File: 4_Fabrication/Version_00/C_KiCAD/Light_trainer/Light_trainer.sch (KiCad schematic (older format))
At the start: 25 parts, among them SW1 SW_Push, SW2 SW_Push, SW3 SW_Push, SW4 SW_Push, U1 LTC3525-5, U2 ESP32-DevKitC-32D

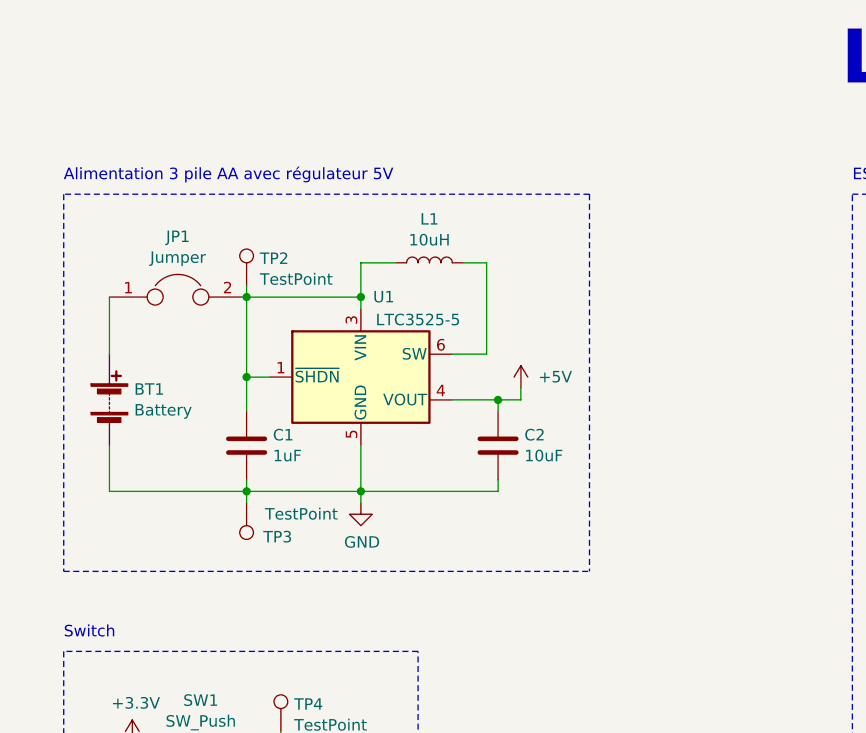
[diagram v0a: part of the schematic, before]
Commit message: placement + routage
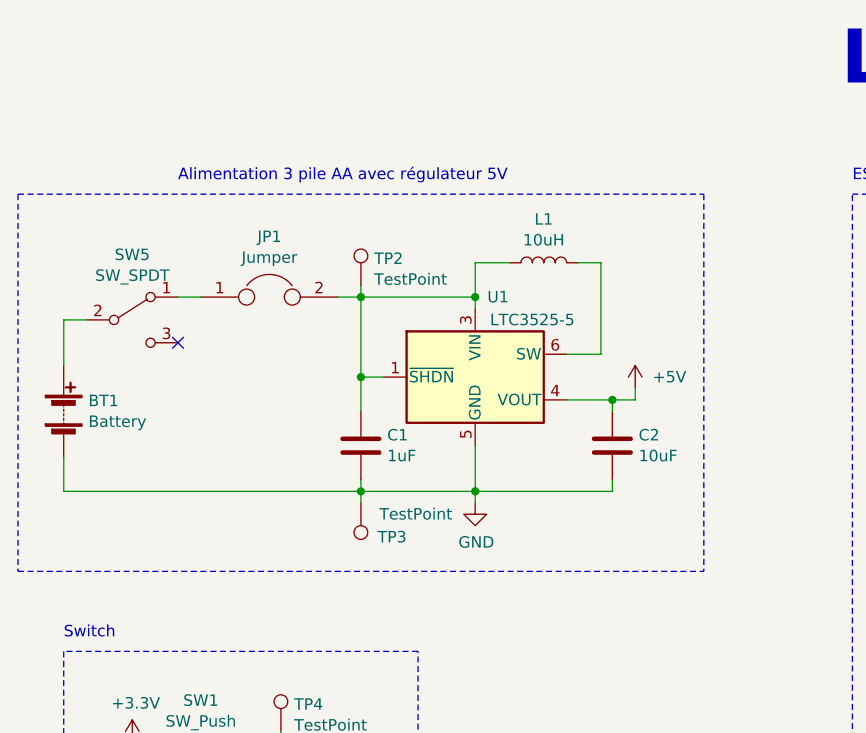
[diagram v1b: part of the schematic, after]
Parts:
- added SW5: SW_SPDT, Work_Forestier:C&K-1101M2S5CQE2, symbol Switch:SW_SPDT
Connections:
- net at BT1.1 (+): now also SW5.2 (B); no longer JP1.1
- new net: JP1.1, SW5.1 (A)
- no-connect marks 31 -> 32
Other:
- moved on the sheet: BT1, C1, C2, JP1, L1, TP2, TP3, U1
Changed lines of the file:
@@
 L Device:Battery BT1
 U 1 1 613C716D
-P 1200 2400
-F 0 "BT1" H 1308 2446 50  0000 L CNN
-F 1 "Battery" H 1308 2355 50  0000 L CNN
-F 2 "Work_Forestier:BatteryHolder_Keystone_2464_3xAA" V 1200 2460 50  0001 C CNN
-F 3 "~" V 1200 2460 50  0001 C CNN
-	1    1200 2400
+P 1000 2450
+F 0 "BT1" H 1108 2496 50  0000 L CNN
+F 1 "Battery" H 1108 2405 50  0000 L CNN
+F 2 "Work_Forestier:BatteryHolder_Keystone_2464_3xAA" V 1000 2510 50  0001 C CNN
+F 3 "~" V 1000 2510 50  0001 C CNN
+	1    1000 2450
 	1    0    0    -1
 $EndComp
@@
 L Regulator_Switching:LTC3525-5 U1
 U 1 1 613E4BD4
-P 2300 2300
-F 0 "U1" H 2400 2650 50  0000 C CNN
-F 1 "LTC3525-5" H 2550 2550 50  0000 C CNN
-F 2 "Package_TO_SOT_SMD:SOT-363_SC-70-6" H 2350 2050 50  0001 L CNN
-F 3 "https://www.analog.com/media/en/technical-documentation/data-sheets/3525fc.pdf" H 2300 2300 50  0001 C CNN
-	1    2300 2300
-	1    0    0    -1
-$EndComp
-Wire Wire Line
-	1800 2300 1900 2300
+P 2800 2300
+F 0 "U1" H 2900 2650 50  0000 C CNN
+F 1 "LTC3525-5" H 3050 2550 50  0000 C CNN
+F 2 "Package_TO_SOT_SMD:SOT-363_SC-70-6" H 2850 2050 50  0001 L CNN
+F 3 "https://www.analog.com/media/en/technical-documentation/data-sheets/3525fc.pdf" H 2800 2300 50  0001 C CNN
+	1    2800 2300
+	1    0    0    -1
+$EndComp
+Wire Wire Line
+	2300 2300 2400 2300
 $Comp
 L Device:L L1
 U 1 1 613E7FA8
-P 2600 1800
-F 0 "L1" V 2790 1800 50  0000 C CNN
-F 1 "10uH" V 2699 1800 50  0000 C CNN
-F 2 "Inductor_SMD:L_1210_3225Metric" H 2600 1800 50  0001 C CNN
-F 3 "~" H 2600 1800 50  0001 C CNN
-	1    2600 1800
+P 3100 1800
+F 0 "L1" V 3290 1800 50  0000 C CNN
+F 1 "10uH" V 3199 1800 50  0000 C CNN
+F 2 "Inductor_SMD:L_1210_3225Metric" H 3100 1800 50  0001 C CNN
+F 3 "~" H 3100 1800 50  0001 C CNN
+	1    3100 1800
 	0    -1   -1   0
 $EndComp
 Wire Wire Line
-	2850 1800 2850 2200
-Wire Wire Line
-	2850 2200 2700 2200
+	3350 1800 3350 2200
+Wire Wire Line
+	3350 2200 3200 2200
 $Comp
 L Device:C C2
 U 1 1 613EB1F1
-P 2900 2600
-F 0 "C2" H 3015 2646 50  0000 L CNN
-F 1 "10uF" H 3015 2555 50  0000 L CNN
-F 2 "Capacitor_SMD:C_0805_2012Metric" H 2938 2450 50  0001 C CNN
-F 3 "~" H 2900 2600 50  0001 C CNN
-	1    2900 2600
-	1    0    0    -1
-$EndComp
-Wire Wire Line
-	2900 2400 2900 2450
-Wire Wire Line
-	2700 2400 2900 2400
-Wire Wire Line
-	2900 2400 3000 2400
-Connection ~ 2900 2400
-Wire Wire Line
-	2300 2600 2300 2800
-Wire Wire Line
-	2300 2800 2900 2800
-Wire Wire Line
-	2900 2800 2900 2750
+P 3400 2600
+F 0 "C2" H 3515 2646 50  0000 L CNN
+F 1 "10uF" H 3515 2555 50  0000 L CNN
+F 2 "Capacitor_SMD:C_0805_2012Metric" H 3438 2450 50  0001 C CNN
+F 3 "~" H 3400 2600 50  0001 C CNN
+	1    3400 2600
+	1    0    0    -1
+$EndComp
+Wire Wire Line
+	3400 2400 3400 2450
+Wire Wire Line
+	3200 2400 3400 2400
+Wire Wire Line
+	3400 2400 3500 2400
+Connection ~ 3400 2400
+Wire Wire Line
+	2800 2600 2800 2800
+Wire Wire Line
+	2800 2800 3400 2800
+Wire Wire Line
+	3400 2800 3400 2750
 $Comp
 L Device:C C1
 U 1 1 613F1363
-P 1800 2600
-F 0 "C1" H 1915 2646 50  0000 L CNN
-F 1 "1uF" H 1915 2555 50  0000 L CNN
-F 2 "Capacitor_SMD:C_0805_2012Metric" H 1838 2450 50  0001 C CNN
-F 3 "~" H 1800 2600 50  0001 C CNN
-	1    1800 2600
-	1    0    0    -1
-$EndComp
-Wire Wire Line
-	2300 2800 1800 2800
-Wire Wire Line
-	1800 2800 1800 2750
-Connection ~ 2300 2800
-Wire Wire Line
-	1800 2450 1800 2300
-Wire Wire Line
-	2300 1800 2450 1800
-Wire Wire Line
-	2750 1800 2850 1800
-Wire Wire Line
-	1200 2600 1200 2800
-Wire Notes Line
-	1000 3150 3300 3150
-Wire Notes Line
-	3300 1500 1000 1500
+P 2300 2600
+F 0 "C1" H 2415 2646 50  0000 L CNN
+F 1 "1uF" H 2415 2555 50  0000 L CNN
+F 2 "Capacitor_SMD:C_0805_2012Metric" H 2338 2450 50  0001 C CNN
+F 3 "~" H 2300 2600 50  0001 C CNN
+	1    2300 2600
+	1    0    0    -1
+$EndComp
+Wire Wire Line
+	2800 2800 2300 2800
+Wire Wire Line
+	2300 2800 2300 2750
+Connection ~ 2800 2800
+Wire Wire Line
+	2300 2450 2300 2300
+Wire Wire Line
+	2800 1800 2950 1800
+Wire Wire Line
+	3250 1800 3350 1800
 $Comp
 L Light_trainer-rescue:+5V-power #PWR013
@@
 L Light_trainer-rescue:+5V-power #PWR08
 U 1 1 61414884
-P 3000 2350
-F 0 "#PWR08" H 3000 2200 50  0001 C CNN
-F 1 "+5V" H 3150 2400 50  0000 C CNN
-F 2 "" H 3000 2350 50  0001 C CNN
-F 3 "" H 3000 2350 50  0001 C CNN
-	1    3000 2350
-	1    0    0    -1
-$EndComp
-Wire Wire Line
-	3000 2350 3000 2400
+P 3500 2350
+F 0 "#PWR08" H 3500 2200 50  0001 C CNN
+F 1 "+5V" H 3650 2400 50  0000 C CNN
+F 2 "" H 3500 2350 50  0001 C CNN
+F 3 "" H 3500 2350 50  0001 C CNN
+	1    3500 2350
+	1    0    0    -1
+$EndComp
+Wire Wire Line
+	3500 2350 3500 2400
 $Comp
 L Light_trainer-rescue:GND-power #PWR05
 U 1 1 61415E58
-P 2300 2850
-F 0 "#PWR05" H 2300 2600 50  0001 C CNN
-F 1 "GND" H 2305 2677 50  0000 C CNN
-F 2 "" H 2300 2850 50  0001 C CNN
-F 3 "" H 2300 2850 50  0001 C CNN
-	1    2300 2850
-	1    0    0    -1
-$EndComp
-Wire Wire Line
-	2300 2850 2300 2800
-Wire Notes Line
-	3300 1500 3300 3150
-Wire Notes Line
-	1000 1500 1000 3150
+P 2800 2850
+F 0 "#PWR05" H 2800 2600 50  0001 C CNN
+F 1 "GND" H 2805 2677 50  0000 C CNN
+F 2 "" H 2800 2850 50  0001 C CNN
+F 3 "" H 2800 2850 50  0001 C CNN
+	1    2800 2850
+	1    0    0    -1
+$EndComp
+Wire Wire Line
+	2800 2850 2800 2800
+Wire Notes Line
+	3800 1500 3800 3150
+Wire Notes Line
+	800  1500 800  3150
 $Comp
 L Light_trainer-rescue:+5V-power #PWR017
@@
 L Connector:TestPoint TP2
 U 1 1 6143AF5D
-P 1800 1900
-F 0 "TP2" H 1858 2018 50  0000 L CNN
-F 1 "TestPoint" H 1858 1927 50  0000 L CNN
-F 2 "TestPoint:TestPoint_THTPad_2.5x2.5mm_Drill1.2mm" H 2000 1900 50  0001 C CNN
-F 3 "~" H 2000 1900 50  0001 C CNN
-F 4 "~" H 1800 1900 50  0001 C CNN "Fournisseur"
-F 5 "~" H 1800 1900 50  0001 C CNN "Prix total"
-F 6 "~" H 1800 1900 50  0001 C CNN "prix unité"
-	1    1800 1900
+P 2300 1900
+F 0 "TP2" H 2358 2018 50  0000 L CNN
+F 1 "TestPoint" H 2358 1927 50  0000 L CNN
+F 2 "TestPoint:TestPoint_THTPad_2.5x2.5mm_Drill1.2mm" H 2500 1900 50  0001 C CNN
+F 3 "~" H 2500 1900 50  0001 C CNN
+F 4 "~" H 2300 1900 50  0001 C CNN "Fournisseur"
+F 5 "~" H 2300 1900 50  0001 C CNN "Prix total"
+F 6 "~" H 2300 1900 50  0001 C CNN "prix unité"
+	1    2300 1900
 	1    0    0    -1
 $EndComp
@@
 L Connector:TestPoint TP3
 U 1 1 6143D663
-P 1800 2850
-F 0 "TP3" H 1600 3000 50  0000 L CNN
-F 1 "TestPoint" H 1400 2900 50  0000 L CNN
-F 2 "TestPoint:TestPoint_THTPad_2.5x2.5mm_Drill1.2mm" H 2000 2850 50  0001 C CNN
-F 3 "~" H 2000 2850 50  0001 C CNN
-F 4 "~" H 1800 2850 50  0001 C CNN "Fournisseur"
-F 5 "~" H 1800 2850 50  0001 C CNN "Prix total"
-F 6 "~" H 1800 2850 50  0001 C CNN "prix unité"
-	1    1800 2850
+P 2300 2850
+F 0 "TP3" H 2100 3000 50  0000 L CNN
+F 1 "TestPoint" H 1900 2900 50  0000 L CNN
+F 2 "TestPoint:TestPoint_THTPad_2.5x2.5mm_Drill1.2mm" H 2500 2850 50  0001 C CNN
+F 3 "~" H 2500 2850 50  0001 C CNN
+F 4 "~" H 2300 2850 50  0001 C CNN "Fournisseur"
+F 5 "~" H 2300 2850 50  0001 C CNN "Prix total"
+F 6 "~" H 2300 2850 50  0001 C CNN "prix unité"
+	1    2300 2850
 	-1   0    0    1
 $EndComp
 Wire Wire Line
-	1800 2800 1800 2850
+	2300 2800 2300 2850
 Wire Wire Line
 	6050 2950 6250 2950
@@
 Text Notes 4450 1450 0    50   ~ 0
 ESP DEVKIT C\n
-Text Notes 1000 1450 0    50   ~ 0
+Text Notes 1500 1450 0    50   ~ 0
 Alimentation 3 pile AA avec régulateur 5V\n
 Text Notes 4500 4550 0    50   ~ 0
@@
 L Device:Jumper JP1
 U 1 1 614DCE52
-P 1500 1950
-F 0 "JP1" H 1500 2214 50  0000 C CNN
-F 1 "Jumper" H 1500 2123 50  0000 C CNN
-F 2 "Jumper:SolderJumper-2_P1.3mm_Open_Pad1.0x1.5mm" H 1500 1950 50  0001 C CNN
-F 3 "~" H 1500 1950 50  0001 C CNN
-F 4 "~" H 1500 1950 50  0001 C CNN "Fournisseur"
-F 5 "~" H 1500 1950 50  0001 C CNN "Prix total"
-F 6 "~" H 1500 1950 50  0001 C CNN "prix unité"
-	1    1500 1950
-	1    0    0    -1
-$EndComp
-Wire Wire Line
-	2300 1800 2300 1950
-Wire Wire Line
-	1800 2300 1800 1950
-Connection ~ 1800 2300
-Wire Wire Line
-	1800 1950 1800 1900
-Connection ~ 1800 1950
-Wire Wire Line
-	1200 1950 1200 2200
-Wire Wire Line
-	1800 1950 2300 1950
+P 1900 1950
+F 0 "JP1" H 1900 2214 50  0000 C CNN
+F 1 "Jumper" H 1900 2123 50  0000 C CNN
+F 2 "Jumper:SolderJumper-2_P1.3mm_Open_Pad1.0x1.5mm" H 1900 1950 50  0001 C CNN
+F 3 "~" H 1900 1950 50  0001 C CNN
+F 4 "~" H 1900 1950 50  0001 C CNN "Fournisseur"
+F 5 "~" H 1900 1950 50  0001 C CNN "Prix total"
+F 6 "~" H 1900 1950 50  0001 C CNN "prix unité"
+	1    1900 1950
+	1    0    0    -1
+$EndComp
+Wire Wire Line
+	2800 1800 2800 1950
+Wire Wire Line
+	2300 2300 2300 1950
+Connection ~ 2300 2300
+Wire Wire Line
+	2300 1950 2300 1900
 Connection ~ 2300 1950
 Wire Wire Line
-	2300 1950 2300 2000
-Wire Wire Line
-	1200 2800 1800 2800
-Connection ~ 1800 2800
+	2300 1950 2800 1950
+Connection ~ 2800 1950
+Wire Wire Line
+	2800 1950 2800 2000
+Connection ~ 2300 2800
+$Comp
+L Switch:SW_SPDT SW5
+U 1 1 61410395
+P 1300 2050
+F 0 "SW5" H 1300 2335 50  0000 C CNN
+F 1 "SW_SPDT" H 1300 2244 50  0000 C CNN
+F 2 "Work_Forestier:C&K-1101M2S5CQE2" H 1300 2050 50  0001 C CNN
+F 3 "https://www.ckswitches.com/media/1429/1000.pdf" H 1300 2050 50  0001 C CNN
+	1    1300 2050
+	1    0    0    -1
+$EndComp
+Wire Wire Line
+	1000 2800 2300 2800
+Wire Wire Line
+	1000 2050 1100 2050
+NoConn ~ 1500 2150
+Wire Notes Line
+	800  1500 3800 1500
+Wire Notes Line
+	800  3150 3800 3150
+Wire Wire Line
+	2200 1950 2300 1950
+Wire Wire Line
+	1600 1950 1500 1950
+Wire Wire Line
+	1000 2650 1000 2800
+Wire Wire Line
+	1000 2250 1000 2050
 $EndSCHEMATC
